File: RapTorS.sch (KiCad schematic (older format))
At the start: 22 parts, among them J1 Molex 48037-2200, J2 TestPoint, J3 TestPoint, J4 TestPoint, J5 TestPoint, J6 TestPoint, U1 PIC16LF1454-I_ML, U2 TLV71333PDBV, U3 E07-M1101S

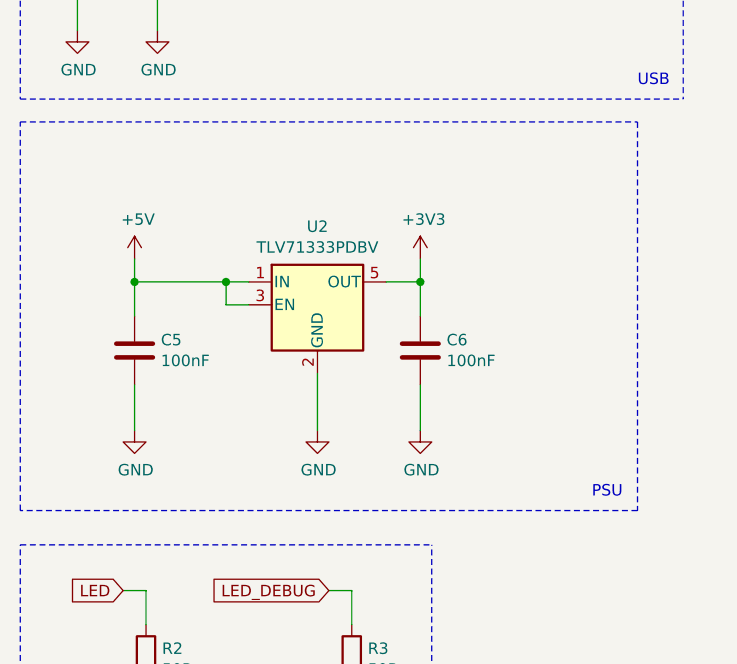
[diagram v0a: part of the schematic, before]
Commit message: placement second step
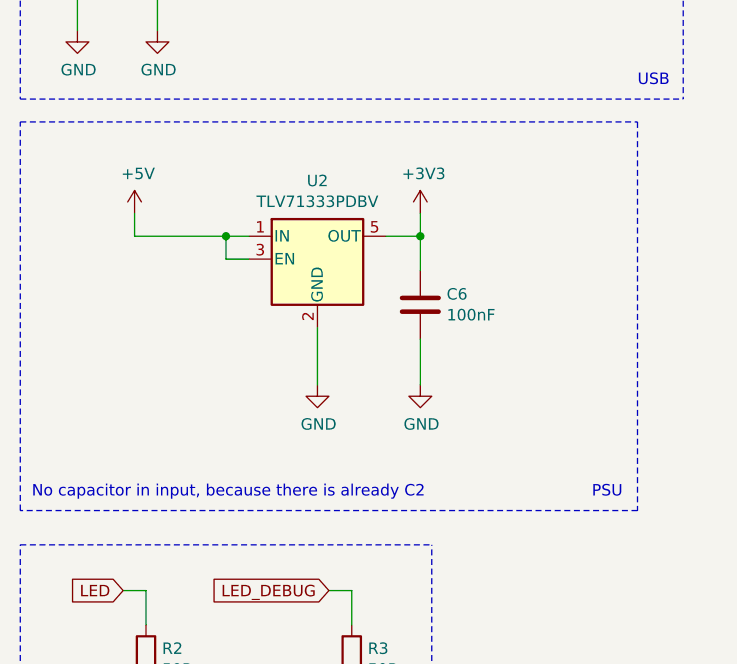
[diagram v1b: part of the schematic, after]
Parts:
- removed C5: 100nF, Capacitors_SMD:C_0805, symbol RapTorS-rescue:C-device
- J2: footprint Connectors_TestPoints:Test_Point_Pad_1.5x1.5mm -> Connectors_TestPoints:Test_Point_Pad_d1.5mm
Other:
- note added: "No capacitor in input, because there is already C2"
- moved on the sheet: C6, U2
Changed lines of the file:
@@
-$EndComp
-$Comp
-L RapTorS-rescue:C-device C5
-U 1 1 5B62F7D7
-P 1500 3800
-F 0 "C5" H 1615 3846 50  0000 L CNN
-F 1 "100nF" H 1615 3755 50  0000 L CNN
-F 2 "Capacitors_SMD:C_0805" H 1538 3650 50  0001 C CNN
-F 3 "" H 1500 3800 50  0001 C CNN
-	1    1500 3800
-	1    0    0    -1
 $EndComp
 $Comp
@@
 L RapTorS-rescue:TLV71333PDBV-regul U2
 U 1 1 5B6396D9
-P 2300 3600
-F 0 "U2" H 2300 3942 50  0000 C CNN
-F 1 "TLV71333PDBV" H 2300 3851 50  0000 C CNN
-F 2 "TO_SOT_Packages_SMD:SOT-23-5" H 2300 3925 50  0001 C CIN
-F 3 "http://www.ti.com/lit/ds/symlink/tlv713p.pdf" H 2300 3600 50  0001 C CNN
-	1    2300 3600
+P 2300 3400
+F 0 "U2" H 2300 3742 50  0000 C CNN
+F 1 "TLV71333PDBV" H 2300 3651 50  0000 C CNN
+F 2 "TO_SOT_Packages_SMD:SOT-23-5" H 2300 3725 50  0001 C CIN
+F 3 "http://www.ti.com/lit/ds/symlink/tlv713p.pdf" H 2300 3400 50  0001 C CNN
+	1    2300 3400
 	1    0    0    -1
 $EndComp
@@
 L power:GND #PWR017
 U 1 1 5B68188F
-P 2300 4150
-F 0 "#PWR017" H 2300 3900 50  0001 C CNN
-F 1 "GND" H 2305 3977 50  0000 C CNN
-F 2 "" H 2300 4150 50  0001 C CNN
-F 3 "" H 2300 4150 50  0001 C CNN
-	1    2300 4150
-	1    0    0    -1
-$EndComp
-$Comp
-L power:GND #PWR016
-U 1 1 5B6818B6
-P 1500 4150
-F 0 "#PWR016" H 1500 3900 50  0001 C CNN
-F 1 "GND" H 1505 3977 50  0000 C CNN
-F 2 "" H 1500 4150 50  0001 C CNN
-F 3 "" H 1500 4150 50  0001 C CNN
-	1    1500 4150
-	1    0    0    -1
-$EndComp
-Wire Wire Line
-	1500 4150 1500 3950
-Wire Wire Line
-	1500 3500 1900 3500
-Wire Wire Line
-	2000 3600 1900 3600
-Wire Wire Line
-	1900 3600 1900 3500
-Connection ~ 1900 3500
-Wire Wire Line
-	1900 3500 2000 3500
-Wire Wire Line
-	1500 3500 1500 3650
-Wire Wire Line
-	2300 4150 2300 3900
+P 2300 3950
+F 0 "#PWR017" H 2300 3700 50  0001 C CNN
+F 1 "GND" H 2305 3777 50  0000 C CNN
+F 2 "" H 2300 3950 50  0001 C CNN
+F 3 "" H 2300 3950 50  0001 C CNN
+	1    2300 3950
+	1    0    0    -1
+$EndComp
+Wire Wire Line
+	1500 3300 1900 3300
+Wire Wire Line
+	2000 3400 1900 3400
+Wire Wire Line
+	1900 3400 1900 3300
+Connection ~ 1900 3300
+Wire Wire Line
+	1900 3300 2000 3300
+Wire Wire Line
+	2300 3950 2300 3700
 $Comp
 L power:+5V #PWR012
 U 1 1 5B683BB0
-P 1500 3400
-F 0 "#PWR012" H 1500 3250 50  0001 C CNN
-F 1 "+5V" H 1515 3573 50  0000 C CNN
-F 2 "" H 1500 3400 50  0001 C CNN
-F 3 "" H 1500 3400 50  0001 C CNN
-	1    1500 3400
-	1    0    0    -1
-$EndComp
-Wire Wire Line
-	1500 3500 1500 3400
-Connection ~ 1500 3500
+P 1500 3200
+F 0 "#PWR012" H 1500 3050 50  0001 C CNN
+F 1 "+5V" H 1515 3373 50  0000 C CNN
+F 2 "" H 1500 3200 50  0001 C CNN
+F 3 "" H 1500 3200 50  0001 C CNN
+	1    1500 3200
+	1    0    0    -1
+$EndComp
+Wire Wire Line
+	1500 3300 1500 3200
 $Comp
 L RapTorS-rescue:C-device C6
 U 1 1 5B684462
-P 2750 3800
-F 0 "C6" H 2865 3846 50  0000 L CNN
-F 1 "100nF" H 2865 3755 50  0000 L CNN
-F 2 "Capacitors_SMD:C_0805" H 2788 3650 50  0001 C CNN
-F 3 "" H 2750 3800 50  0001 C CNN
-	1    2750 3800
-	1    0    0    -1
-$EndComp
-Wire Wire Line
-	2600 3500 2750 3500
-Wire Wire Line
-	2750 3500 2750 3650
+P 2750 3600
+F 0 "C6" H 2865 3646 50  0000 L CNN
+F 1 "100nF" H 2865 3555 50  0000 L CNN
+F 2 "Capacitors_SMD:C_0805" H 2788 3450 50  0001 C CNN
+F 3 "" H 2750 3600 50  0001 C CNN
+	1    2750 3600
+	1    0    0    -1
+$EndComp
+Wire Wire Line
+	2600 3300 2750 3300
+Wire Wire Line
+	2750 3300 2750 3450
 $Comp
 L power:GND #PWR018
 U 1 1 5B684DFE
-P 2750 4150
-F 0 "#PWR018" H 2750 3900 50  0001 C CNN
-F 1 "GND" H 2755 3977 50  0000 C CNN
-F 2 "" H 2750 4150 50  0001 C CNN
-F 3 "" H 2750 4150 50  0001 C CNN
-	1    2750 4150
-	1    0    0    -1
-$EndComp
-Wire Wire Line
-	2750 4150 2750 3950
+P 2750 3950
+F 0 "#PWR018" H 2750 3700 50  0001 C CNN
+F 1 "GND" H 2755 3777 50  0000 C CNN
+F 2 "" H 2750 3950 50  0001 C CNN
+F 3 "" H 2750 3950 50  0001 C CNN
+	1    2750 3950
+	1    0    0    -1
+$EndComp
+Wire Wire Line
+	2750 3950 2750 3750
 $Comp
 L power:+3V3 #PWR013
 U 1 1 5B685845
-P 2750 3400
-F 0 "#PWR013" H 2750 3250 50  0001 C CNN
-F 1 "+3V3" H 2765 3573 50  0000 C CNN
-F 2 "" H 2750 3400 50  0001 C CNN
-F 3 "" H 2750 3400 50  0001 C CNN
-	1    2750 3400
-	1    0    0    -1
-$EndComp
-Connection ~ 2750 3500
-Wire Wire Line
-	2750 3400 2750 3500
+P 2750 3200
+F 0 "#PWR013" H 2750 3050 50  0001 C CNN
+F 1 "+3V3" H 2765 3373 50  0000 C CNN
+F 2 "" H 2750 3200 50  0001 C CNN
+F 3 "" H 2750 3200 50  0001 C CNN
+	1    2750 3200
+	1    0    0    -1
+$EndComp
+Connection ~ 2750 3300
+Wire Wire Line
+	2750 3200 2750 3300
 Wire Notes Line
 	1000 2800 3700 2800
@@
 F 0 "J2" V 5700 3787 50  0000 L CNN
 F 1 "TestPoint" V 5745 3788 50  0001 L CNN
-F 2 "Connectors_TestPoints:Test_Point_Pad_1.5x1.5mm" H 5900 3600 50  0001 C CNN
+F 2 "Connectors_TestPoints:Test_Point_Pad_d1.5mm" H 5900 3600 50  0001 C CNN
 F 3 "~" H 5900 3600 50  0001 C CNN
 	1    5700 3600
@@
 Wire Notes Line
 	1000 800  3900 800
+Text Notes 1050 4450 0    50   ~ 0
+No capacitor in input, because there is already C2
 $EndSCHEMATC
